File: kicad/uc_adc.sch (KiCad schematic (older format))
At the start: 6 parts, among them U401 TMS320F28388DZWTS

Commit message: begin PCB!! it's amess but IT IS
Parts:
- C429, C432, C433, C436: footprint (none) -> Capacitor_SMD:C_0603_1608Metric
- R436: footprint (none) -> Resistor_SMD:R_0603_1608Metric
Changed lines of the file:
@@
 F 0 "C433" V 8350 4400 60  0000 R CNN
 F 1 "2.2uF" V 8150 4400 50  0000 R CNN
-F 2 "" H 8200 4150 50  0001 C CNN
+F 2 "Capacitor_SMD:C_0603_1608Metric" H 8200 4150 50  0001 C CNN
 F 3 "" H 8200 4150 50  0001 C CNN
 F 4 "2.2uF" V -2300 3250 60  0001 C CNN "ValueDisplayed"
@@
 F 0 "C436" V 7645 4040 60  0000 R CNN
 F 1 "1uF" V 7547 4040 50  0000 R CNN
-F 2 "" H 7550 4150 50  0001 C CNN
+F 2 "Capacitor_SMD:C_0603_1608Metric" H 7550 4150 50  0001 C CNN
 F 3 "" H 7550 4150 50  0001 C CNN
 F 4 "1uF" V -6850 3450 60  0001 C CNN "ValueDisplayed"
@@
 F 0 "C429" V 7145 4040 60  0000 R CNN
 F 1 "22uF" V 7047 4040 50  0000 R CNN
-F 2 "" H 7050 4150 50  0001 C CNN
+F 2 "Capacitor_SMD:C_0603_1608Metric" H 7050 4150 50  0001 C CNN
 F 3 "" H 7050 4150 50  0001 C CNN
 F 4 "22uF" V -2350 -1650 60  0001 C CNN "ValueDisplayed"
@@
 F 0 "C432" V 8695 4259 60  0000 L CNN
 F 1 "0.1uF" V 8597 4259 50  0000 L CNN
-F 2 "" H 8600 4150 50  0001 C CNN
+F 2 "Capacitor_SMD:C_0603_1608Metric" H 8600 4150 50  0001 C CNN
 F 3 "" H 8600 4150 50  0001 C CNN
 F 4 "0.1uF" V -1500 3250 60  0001 C CNN "ValueDisplayed"
@@
 F 0 "R436" H 7850 3241 60  0000 C CNN
 F 1 "1k" H 7850 3347 60  0000 C CNN
-F 2 "" H 7850 3450 50  0001 C CNN
+F 2 "Resistor_SMD:R_0603_1608Metric" H 7850 3450 50  0001 C CNN
 F 3 "" H 7850 3450 50  0001 C CNN
 F 4 "" V -2150 650 60  0001 C CNN "ValueDisplayed"

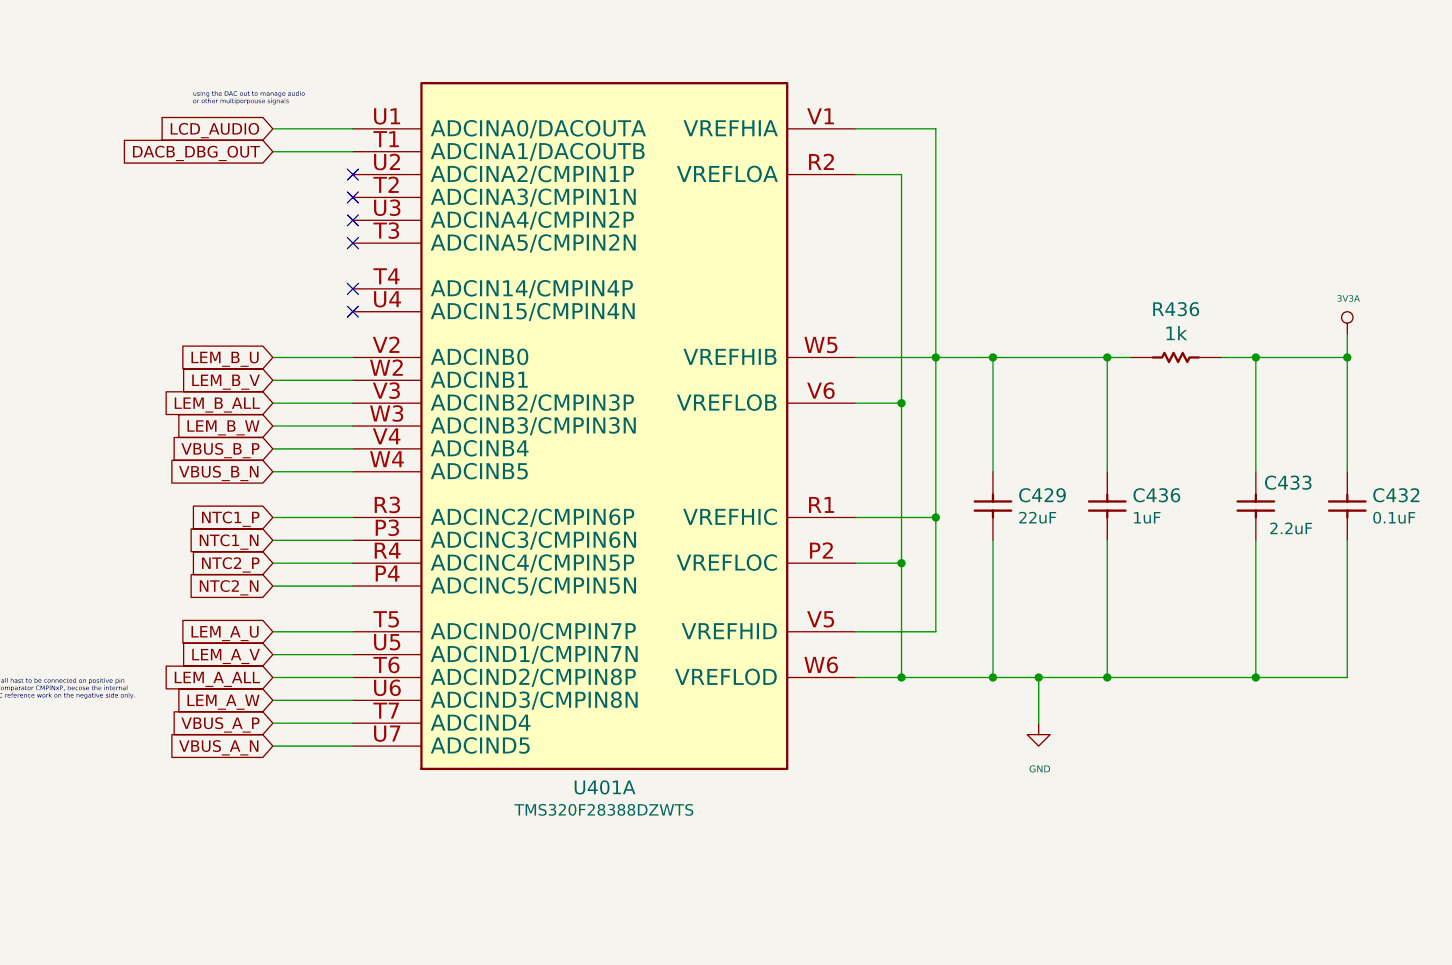
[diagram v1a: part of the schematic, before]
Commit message: I've passed all footprin to layout BUT...
I've passed all, first glance... I need to confirm in details a lot of
things. The objetive for these is to have an aproximation of the size
I'll need to make the board.. then I choose the final detailed footprint
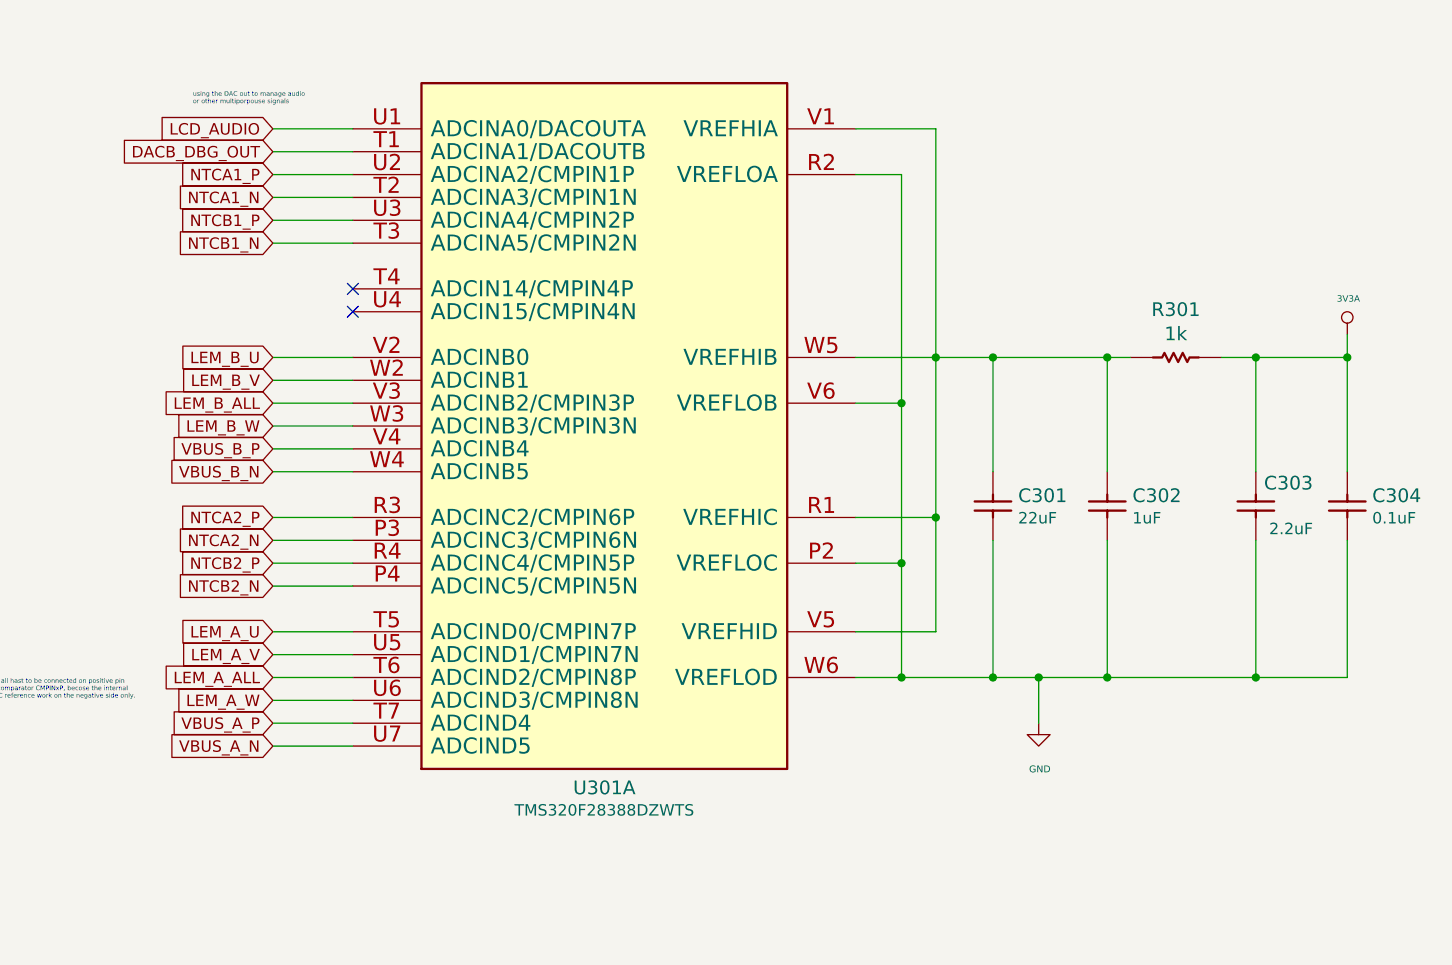
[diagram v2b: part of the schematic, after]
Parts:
- C301: renamed from C429; footprint Capacitor_SMD:C_0603_1608Metric -> servo:C_0603_1608Metric
- C302: renamed from C436; footprint Capacitor_SMD:C_0603_1608Metric -> servo:C_0603_1608Metric
- C303: renamed from C433; footprint Capacitor_SMD:C_0603_1608Metric -> servo:C_0603_1608Metric
- C304: renamed from C432; footprint Capacitor_SMD:C_0603_1608Metric -> servo:C_0603_1608Metric
- U301: renamed from U401; footprint (none) -> servo:BGA337CP80_19X19_1600X1600X140B50N
- renumbered R436 to R301
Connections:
- net NTCA1_N: now reaches U301.T2 (ADCINA3/CMPIN1N)
- net NTCB1_N: now reaches U301.T3 (ADCINA5/CMPIN2N)
- net NTCA1_P: now reaches U301.U2 (ADCINA2/CMPIN1P)
- net NTCB1_P: now reaches U301.U3 (ADCINA4/CMPIN2P)
- net NTC1_N renamed NTCA2_N
- net NTC1_P renamed NTCA2_P
- net NTC2_N renamed NTCB2_N
- net NTC2_P renamed NTCB2_P
- no-connect marks 6 -> 2
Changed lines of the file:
@@
 $Descr A3 16535 11693
 encoding utf-8
-Sheet 3 18
+Sheet 3 19
 Title "ADC"
 Date "2020-01-09"
@@
 Connection ~ 6650 3650
 $Comp
-L servo:Capacitor C433
+L servo:Capacitor C303
 U 1 1 5DB391B8
 P 8200 4150
-F 0 "C433" V 8350 4400 60  0000 R CNN
+F 0 "C303" V 8350 4400 60  0000 R CNN
 F 1 "2.2uF" V 8150 4400 50  0000 R CNN
-F 2 "Capacitor_SMD:C_0603_1608Metric" H 8200 4150 50  0001 C CNN
+F 2 "servo:C_0603_1608Metric" H 8200 4150 50  0001 C CNN
 F 3 "" H 8200 4150 50  0001 C CNN
 F 4 "2.2uF" V -2300 3250 60  0001 C CNN "ValueDisplayed"
@@
 $EndComp
 $Comp
-L servo:Capacitor C436
+L servo:Capacitor C302
 U 1 1 5DB391B3
 P 7550 4150
-F 0 "C436" V 7645 4040 60  0000 R CNN
+F 0 "C302" V 7645 4040 60  0000 R CNN
 F 1 "1uF" V 7547 4040 50  0000 R CNN
-F 2 "Capacitor_SMD:C_0603_1608Metric" H 7550 4150 50  0001 C CNN
+F 2 "servo:C_0603_1608Metric" H 7550 4150 50  0001 C CNN
 F 3 "" H 7550 4150 50  0001 C CNN
 F 4 "1uF" V -6850 3450 60  0001 C CNN "ValueDisplayed"
@@
 $EndComp
 $Comp
-L servo:Capacitor C429
+L servo:Capacitor C301
 U 1 1 5DB3916A
 P 7050 4150
-F 0 "C429" V 7145 4040 60  0000 R CNN
+F 0 "C301" V 7145 4040 60  0000 R CNN
 F 1 "22uF" V 7047 4040 50  0000 R CNN
-F 2 "Capacitor_SMD:C_0603_1608Metric" H 7050 4150 50  0001 C CNN
+F 2 "servo:C_0603_1608Metric" H 7050 4150 50  0001 C CNN
 F 3 "" H 7050 4150 50  0001 C CNN
 F 4 "22uF" V -2350 -1650 60  0001 C CNN "ValueDisplayed"
@@
 $EndComp
 $Comp
-L servo:Capacitor C432
+L servo:Capacitor C304
 U 1 1 5DB39165
 P 8600 4150
-F 0 "C432" V 8695 4259 60  0000 L CNN
+F 0 "C304" V 8695 4259 60  0000 L CNN
 F 1 "0.1uF" V 8597 4259 50  0000 L CNN
-F 2 "Capacitor_SMD:C_0603_1608Metric" H 8600 4150 50  0001 C CNN
+F 2 "servo:C_0603_1608Metric" H 8600 4150 50  0001 C CNN
 F 3 "" H 8600 4150 50  0001 C CNN
 F 4 "0.1uF" V -1500 3250 60  0001 C CNN "ValueDisplayed"
@@
 $EndComp
 $Comp
-L servo:3V3A #PWR0416
+L servo:3V3A #PWR0302
 U 1 1 5E5CB351
 P 8600 3350
-F 0 "#PWR0416" H 8605 3557 20  0001 C CNN
+F 0 "#PWR0302" H 8605 3557 20  0001 C CNN
 F 1 "3V3A" H 8605 3507 28  0000 C CNN
 F 2 "" H 8600 3350 50  0001 C CNN
@@
 	7050 3950 7050 3450
 $Comp
-L servo:Resistor R436
+L servo:Resistor R301
 U 1 1 5E88CCA6
 P 7850 3450
-F 0 "R436" H 7850 3241 60  0000 C CNN
+F 0 "R301" H 7850 3241 60  0000 C CNN
 F 1 "1k" H 7850 3347 60  0000 C CNN
 F 2 "Resistor_SMD:R_0603_1608Metric" H 7850 3450 50  0001 C CNN
@@
 Wire Wire Line
 	7250 5050 7250 4850
-$Comp
-L servo:TMS320F28388 U401
-U 1 1 5DB3916E
-P 5350 3750
-F 0 "U401" H 5350 2167 60  0000 C CNN
-F 1 "TMS320F28388DZWTS" H 5350 2069 50  0000 C CNN
-F 2 "" H 5350 3750 50  0001 C CNN
-F 3 "../doc/datasheets/tms320f28388d_datasheet.pdf" H 5350 3750 50  0001 C CNN
-F 4 "TMS320F28388DZWTS" V -1450 -350 60  0001 C CNN "PartNumber"
-	1    5350 3750
-	1    0    0    -1
-$EndComp
 Wire Wire Line
 	4250 5050 3900 5050
@@
 Wire Wire Line
 	3900 3950 4250 3950
-Text GLabel 3900 4150 0    50   Input ~ 0
-NTC1_P
-Text GLabel 3900 4250 0    50   Input ~ 0
-NTC1_N
 Text GLabel 3900 4350 0    50   Input ~ 0
-NTC2_P
+NTCB2_P
 Text GLabel 3900 4450 0    50   Input ~ 0
-NTC2_N
+NTCB2_N
 Wire Wire Line
 	3900 4150 4250 4150
@@
 AR Path="/5DCD812E/5E9C32E8" Ref="#PWR?"  Part="1"
 AR Path="/5EAA846A/5E9C32E8" Ref="#PWR?"  Part="1"
-AR Path="/5DD0E9D6/5E9C32E8" Ref="#PWR0109"  Part="1"
-F 0 "#PWR0109" H 7255 4901 20  0001 C CNN
+AR Path="/5DD0E9D6/5E9C32E8" Ref="#PWR0301"  Part="1"
+F 0 "#PWR0301" H 7255 4901 20  0001 C CNN
 F 1 "GND" H 7255 4849 30  0000 C CNN
 F 2 "" H 7250 5050 70  0000 C CNN
@@
 	1    0    0    -1
 $EndComp
-NoConn ~ 4250 2650
-NoConn ~ 4250 2750
-NoConn ~ 4250 2850
-NoConn ~ 4250 2950
 NoConn ~ 4250 3150
 NoConn ~ 4250 3250
+Text GLabel 3900 4150 0    50   Input ~ 0
+NTCA2_P
+Text GLabel 3900 4250 0    50   Input ~ 0
+NTCA2_N
+Text GLabel 3900 2850 0    50   Input ~ 0
+NTCB1_P
+Text GLabel 3900 2950 0    50   Input ~ 0
+NTCB1_N
+Text GLabel 3900 2650 0    50   Input ~ 0
+NTCA1_P
+Text GLabel 3900 2750 0    50   Input ~ 0
+NTCA1_N
+$Comp
+L servo:TMS320F28388 U301
+U 1 1 5DB3916E
+P 5350 3750
+F 0 "U301" H 5350 2167 60  0000 C CNN
+F 1 "TMS320F28388DZWTS" H 5350 2069 50  0000 C CNN
+F 2 "servo:BGA337CP80_19X19_1600X1600X140B50N" H 5350 3750 50  0001 C CNN
+F 3 "../doc/datasheets/tms320f28388d_datasheet.pdf" H 5350 3750 50  0001 C CNN
+F 4 "TMS320F28388DZWTS" V -1450 -350 60  0001 C CNN "PartNumber"
+	1    5350 3750
+	1    0    0    -1
+$EndComp
+Wire Wire Line
+	4250 2650 3900 2650
+Wire Wire Line
+	3900 2750 4250 2750
+Wire Wire Line
+	4250 2850 3900 2850
+Wire Wire Line
+	3900 2950 4250 2950
 $EndSCHEMATC
